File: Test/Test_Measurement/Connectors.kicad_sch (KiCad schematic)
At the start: 3 parts, among them J2 Conn_01x02_Socket, J3 Conn_01x03_Socket, J4 Conn_01x02_Socket

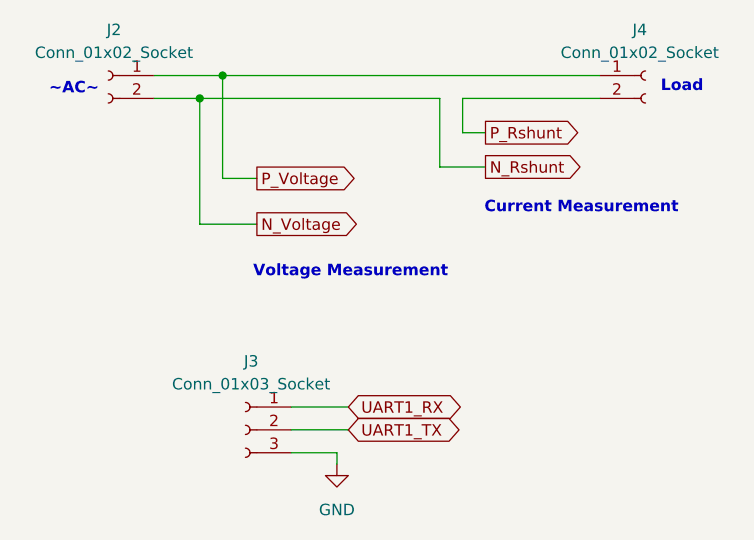
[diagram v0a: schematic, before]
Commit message: Update PCB
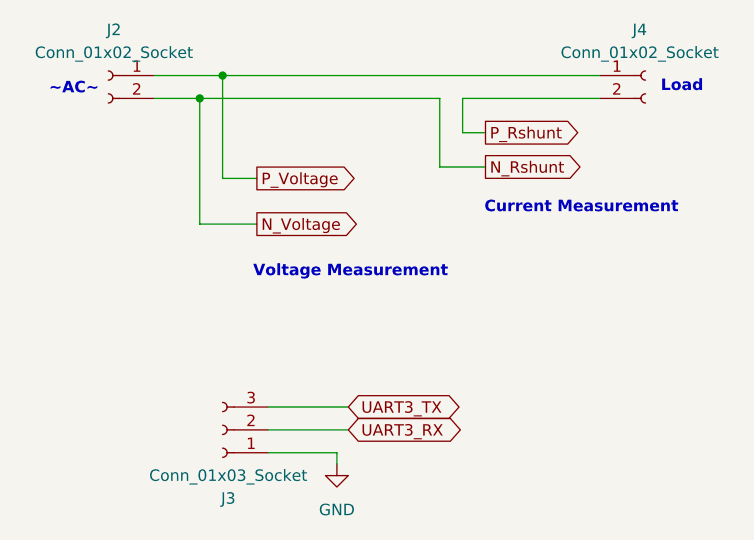
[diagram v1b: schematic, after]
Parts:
- J2, J4: footprint Connector_Phoenix_MC:PhoenixContact_MC_1,5_2-G-3.81_1x02_P3.81mm_Horizontal -> Connector_Phoenix_MC_HighVoltage:PhoenixContact_MC_1,5_2-G-5.08_1x02_P5.08mm_Horizontal
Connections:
- net UART1_RX is gone; now on net GND: J3.1 (Pin_1)
- net GND: no longer J3.3 (Pin_3)
- net UART1_TX renamed UART3_RX
- new net UART3_TX: J3.3 (Pin_3)
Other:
- moved on the sheet: J3
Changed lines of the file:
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@@
-	(wire
-		(pts
-			(xy 100.33 102.87) (xy 106.68 102.87)
-		)
-		(stroke
-			(width 0)
-			(type default)
-		)
-	)
 	(wire
 		(pts
@@
 	(wire
 		(pts
-			(xy 100.33 105.41) (xy 106.68 105.41)
+			(xy 97.79 105.41) (xy 106.68 105.41)
 		)
 		(stroke
@@
 	(wire
 		(pts
+			(xy 119.38 68.58) (xy 134.62 68.58)
+		)
+		(stroke
+			(width 0)
+			(type default)
+		)
+	)
+	(wire
+		(pts
+			(xy 92.71 77.47) (xy 92.71 66.04)
+		)
+		(stroke
+			(width 0)
+			(type default)
+		)
+	)
+	(wire
+		(pts
+			(xy 96.52 82.55) (xy 90.17 82.55)
+		)
+		(stroke
+			(width 0)
+			(type default)
+		)
+	)
+	(wire
+		(pts
+			(xy 85.09 68.58) (xy 90.17 68.58)
+		)
+		(stroke
+			(width 0)
+			(type default)
+		)
+	)
+	(wire
+		(pts
+			(xy 116.84 76.2) (xy 116.84 68.58)
+		)
+		(stroke
+			(width 0)
+			(type default)
+		)
+	)
+	(wire
+		(pts
+			(xy 119.38 68.58) (xy 119.38 72.39)
+		)
+		(stroke
+			(width 0)
+			(type default)
+		)
+	)
+	(wire
+		(pts
+			(xy 119.38 72.39) (xy 121.92 72.39)
+		)
+		(stroke
+			(width 0)
+			(type default)
+		)
+	)
+	(wire
+		(pts
+			(xy 116.84 68.58) (xy 90.17 68.58)
+		)
+		(stroke
+			(width 0)
+			(type default)
+		)
+	)
+	(wire
+		(pts
 			(xy 92.71 66.04) (xy 134.62 66.04)
 		)
@@
 	(wire
 		(pts
-			(xy 92.71 77.47) (xy 92.71 66.04)
-		)
-		(stroke
-			(width 0)
-			(type default)
-		)
-	)
-	(wire
-		(pts
-			(xy 96.52 82.55) (xy 90.17 82.55)
-		)
-		(stroke
-			(width 0)
-			(type default)
-		)
-	)
-	(wire
-		(pts
-			(xy 85.09 68.58) (xy 90.17 68.58)
-		)
-		(stroke
-			(width 0)
-			(type default)
-		)
-	)
-	(wire
-		(pts
-			(xy 116.84 76.2) (xy 116.84 68.58)
-		)
-		(stroke
-			(width 0)
-			(type default)
-		)
-	)
-	(wire
-		(pts
-			(xy 119.38 68.58) (xy 119.38 72.39)
-		)
-		(stroke
-			(width 0)
-			(type default)
-		)
-	)
-	(wire
-		(pts
-			(xy 119.38 72.39) (xy 121.92 72.39)
-		)
-		(stroke
-			(width 0)
-			(type default)
-		)
-	)
-	(wire
-		(pts
-			(xy 116.84 68.58) (xy 90.17 68.58)
+			(xy 97.79 107.95) (xy 105.41 107.95)
 		)
 		(stroke
@@
 	(wire
 		(pts
-			(xy 119.38 68.58) (xy 134.62 68.58)
+			(xy 97.79 102.87) (xy 106.68 102.87)
 		)
 		(stroke
@@
 		(pts
 			(xy 105.41 107.95) (xy 105.41 109.22)
-		)
-		(stroke
-			(width 0)
-			(type default)
-		)
-	)
-	(wire
-		(pts
-			(xy 100.33 107.95) (xy 105.41 107.95)
 		)
 		(stroke
@@
 		)
 	)
-	(global_label "UART1_RX"
+	(global_label "UART3_RX"
 		(shape bidirectional)
-		(at 106.68 102.87 0)
+		(at 106.68 105.41 0)
 		(fields_autoplaced yes)
 		(effects
@@
 		)
 		(property "Intersheetrefs" "${INTERSHEET_REFS}"
-			(at 120.0898 102.87 0)
+			(at 120.0898 105.41 0)
 			(effects
 				(font
@@
 		)
 	)
-	(global_label "UART1_TX"
+	(global_label "UART3_TX"
 		(shape bidirectional)
-		(at 106.68 105.41 0)
+		(at 106.68 102.87 0)
 		(fields_autoplaced yes)
 		(effects
@@
 		)
 		(property "Intersheetrefs" "${INTERSHEET_REFS}"
-			(at 119.7874 105.41 0)
+			(at 119.7874 102.87 0)
 			(effects
 				(font
@@
 	(symbol
 		(lib_id "Connector:Conn_01x03_Socket")
-		(at 95.25 105.41 0)
-		(mirror y)
+		(at 92.71 105.41 180)
 		(unit 1)
 		(exclude_from_sim no)
@@
 		(on_board yes)
 		(dnp no)
-		(fields_autoplaced yes)
 		(property "Reference" "J3"
-			(at 95.885 97.79 0)
+			(at 93.345 113.03 0)
 			(effects
 				(font
@@
 		)
 		(property "Value" "Conn_01x03_Socket"
-			(at 95.885 100.33 0)
+			(at 93.345 110.49 0)
 			(effects
 				(font
@@
 		)
 		(property "Footprint" "Connector_PinHeader_2.54mm:PinHeader_1x03_P2.54mm_Vertical"
-			(at 95.25 105.41 0)
+			(at 92.71 105.41 0)
 			(effects
 				(font
@@
 		)
 		(property "Datasheet" "~"
-			(at 95.25 105.41 0)
+			(at 92.71 105.41 0)
 			(effects
 				(font
@@
 		)
 		(property "Description" "Generic connector, single row, 01x03, script generated"
-			(at 95.25 105.41 0)
+			(at 92.71 105.41 0)
 			(effects
 				(font
@@
 	(symbol
 		(lib_id "Connector:Conn_01x02_Socket")
+		(at 139.7 66.04 0)
+		(unit 1)
+		(exclude_from_sim no)
+		(in_bom yes)
+		(on_board yes)
+		(dnp no)
+		(property "Reference" "J4"
+			(at 139.065 60.96 0)
+			(effects
+				(font
+					(size 1.27 1.27)
+				)
+			)
+		)
+		(property "Value" "Conn_01x02_Socket"
+			(at 139.065 63.5 0)
+			(effects
+				(font
+					(size 1.27 1.27)
+				)
+			)
+		)
+		(property "Footprint" "Connector_Phoenix_MC_HighVoltage:PhoenixContact_MC_1,5_2-G-5.08_1x02_P5.08mm_Horizontal"
+			(at 139.7 66.04 0)
+			(effects
+				(font
+					(size 1.27 1.27)
+				)
+				(hide yes)
+			)
+		)
+		(property "Datasheet" "~"
+			(at 139.7 66.04 0)
+			(effects
+				(font
+					(size 1.27 1.27)
+				)
+				(hide yes)
+			)
+		)
+		(property "Description" "Generic connector, single row, 01x02, script generated"
+			(at 139.7 66.04 0)
+			(effects
+				(font
+					(size 1.27 1.27)
+				)
+				(hide yes)
+			)
+		)
+		(pin "1"
+		)
+		(pin "2"
+		)
+		(instances
+			(project "Test_Measurement"
+				(path "/cd668239-4ad1-4a5c-94e5-ca757cb83213/26bfcc53-9818-4a7f-ae4f-e41e2e94db76"
+					(reference "J4")
+					(unit 1)
+				)
+			)
+		)
+	)
+	(symbol
+		(lib_id "Connector:Conn_01x02_Socket")
 		(at 80.01 66.04 0)
 		(mirror y)
@@
 			)
 		)
-		(property "Footprint" "Connector_Phoenix_MC:PhoenixContact_MC_1,5_2-G-3.81_1x02_P3.81mm_Horizontal"
+		(property "Footprint" "Connector_Phoenix_MC_HighVoltage:PhoenixContact_MC_1,5_2-G-5.08_1x02_P5.08mm_Horizontal"
 			(at 80.01 66.04 0)
 			(effects
@@
 					(unit 1)
 				)
-			)
-		)
-	)
-	(symbol
-		(lib_id "Connector:Conn_01x02_Socket")
-		(at 139.7 66.04 0)
-		(unit 1)
-		(exclude_from_sim no)
-		(in_bom yes)
-		(on_board yes)
-		(dnp no)
-		(property "Reference" "J4"
-			(at 139.065 60.96 0)
-			(effects
-				(font
-					(size 1.27 1.27)
-				)
-			)
-		)
-		(property "Value" "Conn_01x02_Socket"
-			(at 139.065 63.5 0)
-			(effects
-				(font
-					(size 1.27 1.27)
-				)
-			)
-		)
-		(property "Footprint" "Connector_Phoenix_MC:PhoenixContact_MC_1,5_2-G-3.81_1x02_P3.81mm_Horizontal"
-			(at 139.7 66.04 0)
-			(effects
-				(font
-					(size 1.27 1.27)
-				)
-				(hide yes)
-			)
-		)
-		(property "Datasheet" "~"
-			(at 139.7 66.04 0)
-			(effects
-				(font
-					(size 1.27 1.27)
-				)
-				(hide yes)
-			)
-		)
-		(property "Description" "Generic connector, single row, 01x02, script generated"
-			(at 139.7 66.04 0)
-			(effects
-				(font
-					(size 1.27 1.27)
-				)
-				(hide yes)
-			)
-		)
-		(pin "1"
-		)
-		(pin "2"
-		)
-		(instances
-			(project "Test_Measurement"
-				(path "/cd668239-4ad1-4a5c-94e5-ca757cb83213/26bfcc53-9818-4a7f-ae4f-e41e2e94db76"
-					(reference "J4")
-					(unit 1)
-				)
